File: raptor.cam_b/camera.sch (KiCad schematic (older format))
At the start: 3 parts, among them P1 CONN_01X15, P2 CONN_01X05, P3 CONN_01X16

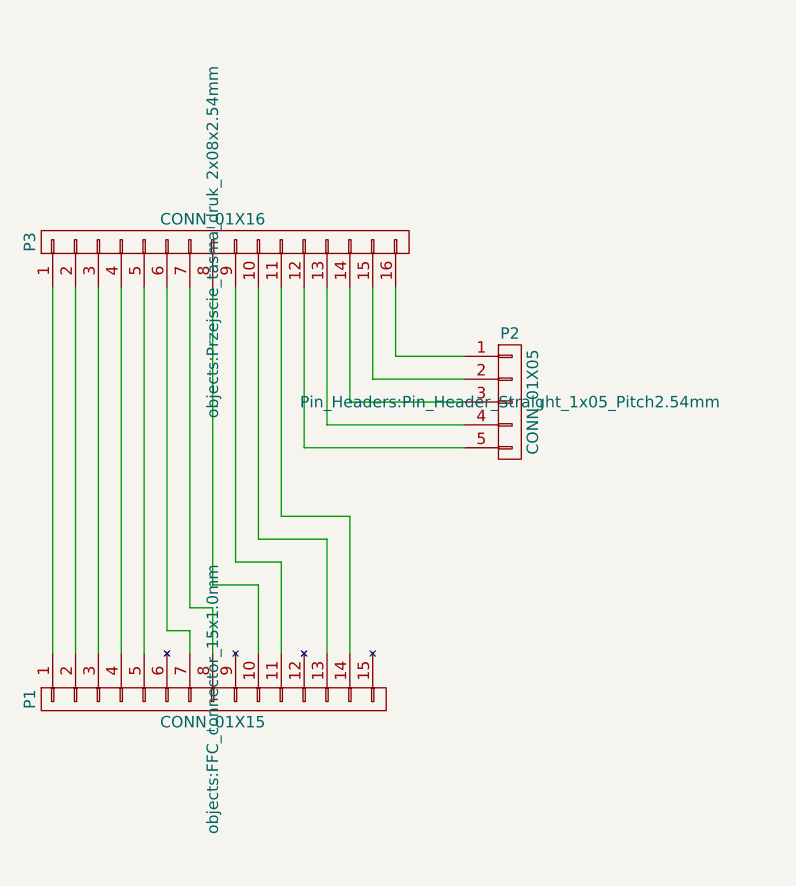
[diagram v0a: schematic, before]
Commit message: Prace nad płytką cd.
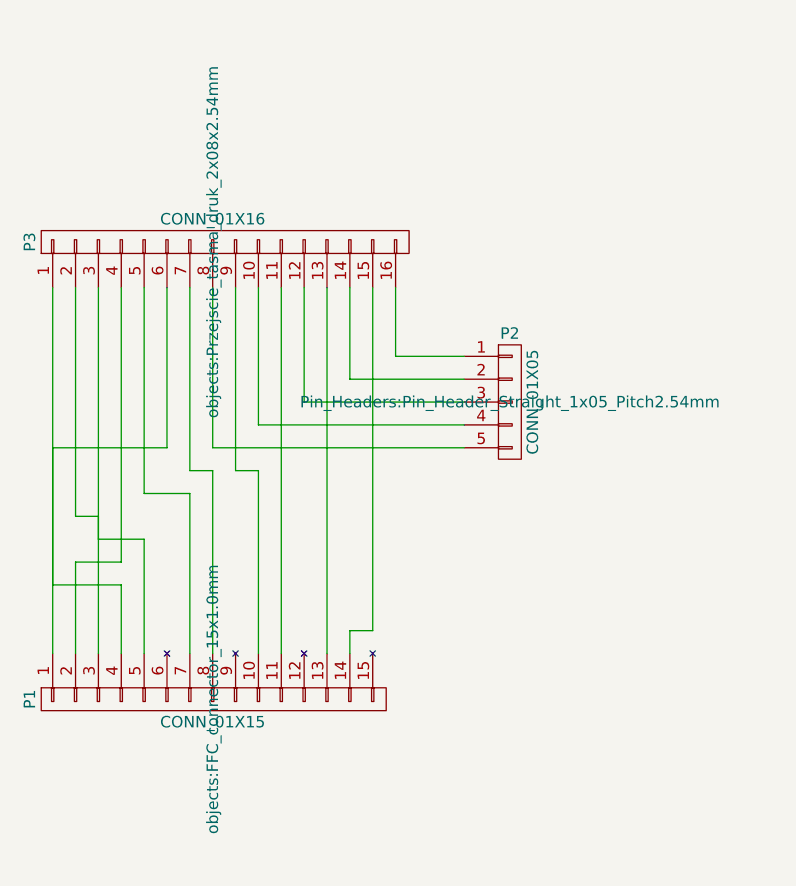
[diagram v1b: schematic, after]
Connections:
- net at P2.2 (P2): now also P3.14 (P14); no longer P3.15 (P15)
- net at P2.3 (P3): now also P3.12 (P12); no longer P3.14 (P14)
- net at P2.4 (P4): now also P3.10 (P10); no longer P3.13 (P13)
- net at P2.5 (P5): now also P3.8 (P8); no longer P3.12 (P12)
- net at P1.1 (P1), P3.1 (P1): now also P1.4 (P4), P3.6 (P6)
- net at P1.10 (P10): now also P3.9 (P9); no longer P3.8 (P8)
- net at P1.11 (P11): now also P3.11 (P11); no longer P3.9 (P9)
- net at P1.13 (P13): now also P3.13 (P13); no longer P3.10 (P10)
- net at P1.14 (P14): now also P3.15 (P15); no longer P3.11 (P11)
- net at P1.2 (P2): now also P3.4 (P4); no longer P3.2 (P2)
- net at P1.3 (P3), P3.3 (P3): now also P1.5 (P5), P3.2 (P2)
- net at P3.5 (P5): now also P1.7 (P7); no longer P1.5 (P5)
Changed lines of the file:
@@
 $EndComp
 Wire Wire Line
-	5300 4300 5300 2700
+	6400 3200 7100 3200
 Wire Wire Line
-	5400 4300 5400 2700
+	7100 3000 6800 3000
 Wire Wire Line
-	5500 4300 5500 2700
+	6800 3000 6800 2700
 Wire Wire Line
-	5600 4300 5600 2700
+	7100 3100 6600 3100
 Wire Wire Line
-	5700 4300 5700 2700
+	6600 3100 6600 2700
 Wire Wire Line
-	5900 4300 5900 4200
+	6400 3200 6400 2700
 Wire Wire Line
-	5900 4200 5800 4200
+	7100 3300 6200 3300
 Wire Wire Line
-	5800 4200 5800 2700
+	6200 3300 6200 2700
 Wire Wire Line
-	6000 4300 6000 4100
+	7100 3400 6000 3400
 Wire Wire Line
-	6000 4100 5900 4100
+	6000 3400 6000 2700
 Wire Wire Line
-	5900 4100 5900 2700
+	6600 4300 6600 4200
 Wire Wire Line
-	6200 4300 6200 4000
+	6600 4200 6700 4200
 Wire Wire Line
-	6200 4000 6000 4000
+	6700 4200 6700 2700
 Wire Wire Line
-	6000 4000 6000 2700
+	6500 4300 6500 2700
 Wire Wire Line
-	6300 4300 6300 3900
+	6300 4300 6300 2700
 Wire Wire Line
-	6300 3900 6100 3900
+	6200 4300 6200 3500
 Wire Wire Line
-	6100 3900 6100 2700
+	6200 3500 6100 3500
 Wire Wire Line
-	6500 4300 6500 3800
+	6100 3500 6100 2700
 Wire Wire Line
-	6500 3800 6200 3800
+	6000 4300 6000 3500
 Wire Wire Line
-	6200 3800 6200 2700
+	6000 3500 5900 3500
 Wire Wire Line
-	6600 4300 6600 3700
+	5900 3500 5900 2700
 Wire Wire Line
-	6600 3700 6300 3700
+	5900 4300 5900 3600
 Wire Wire Line
-	6300 3700 6300 2700
+	5900 3600 5700 3600
 Wire Wire Line
-	6400 2700 6400 3400
+	5700 3600 5700 2700
 Wire Wire Line
-	6400 3400 7100 3400
+	5700 4300 5700 3800
 Wire Wire Line
-	6500 2700 6500 3300
+	5700 3800 5500 3800
 Wire Wire Line
-	6500 3300 7100 3300
+	5500 3800 5500 2700
 Wire Wire Line
-	6600 2700 6600 3200
+	5600 4300 5600 4000
 Wire Wire Line
-	6600 3200 7100 3200
+	5600 4000 5300 4000
 Wire Wire Line
-	6700 2700 6700 3100
+	5300 4000 5300 2700
 Wire Wire Line
-	6700 3100 7100 3100
+	5300 4300 5300 3400
 Wire Wire Line
-	6800 2700 6800 3000
+	5300 3400 5800 3400
 Wire Wire Line
-	6800 3000 7100 3000
+	5800 3400 5800 2700
+Wire Wire Line
+	5400 4300 5400 3900
+Wire Wire Line
+	5400 3900 5600 3900
+Wire Wire Line
+	5600 3900 5600 2700
+Wire Wire Line
+	5500 4300 5500 3700
+Wire Wire Line
+	5500 3700 5400 3700
+Wire Wire Line
+	5400 3700 5400 2700
 $EndSCHEMATC
